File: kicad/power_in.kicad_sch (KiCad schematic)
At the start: 8 parts, among them J1 USB4105-GF-A, U1 CH224K

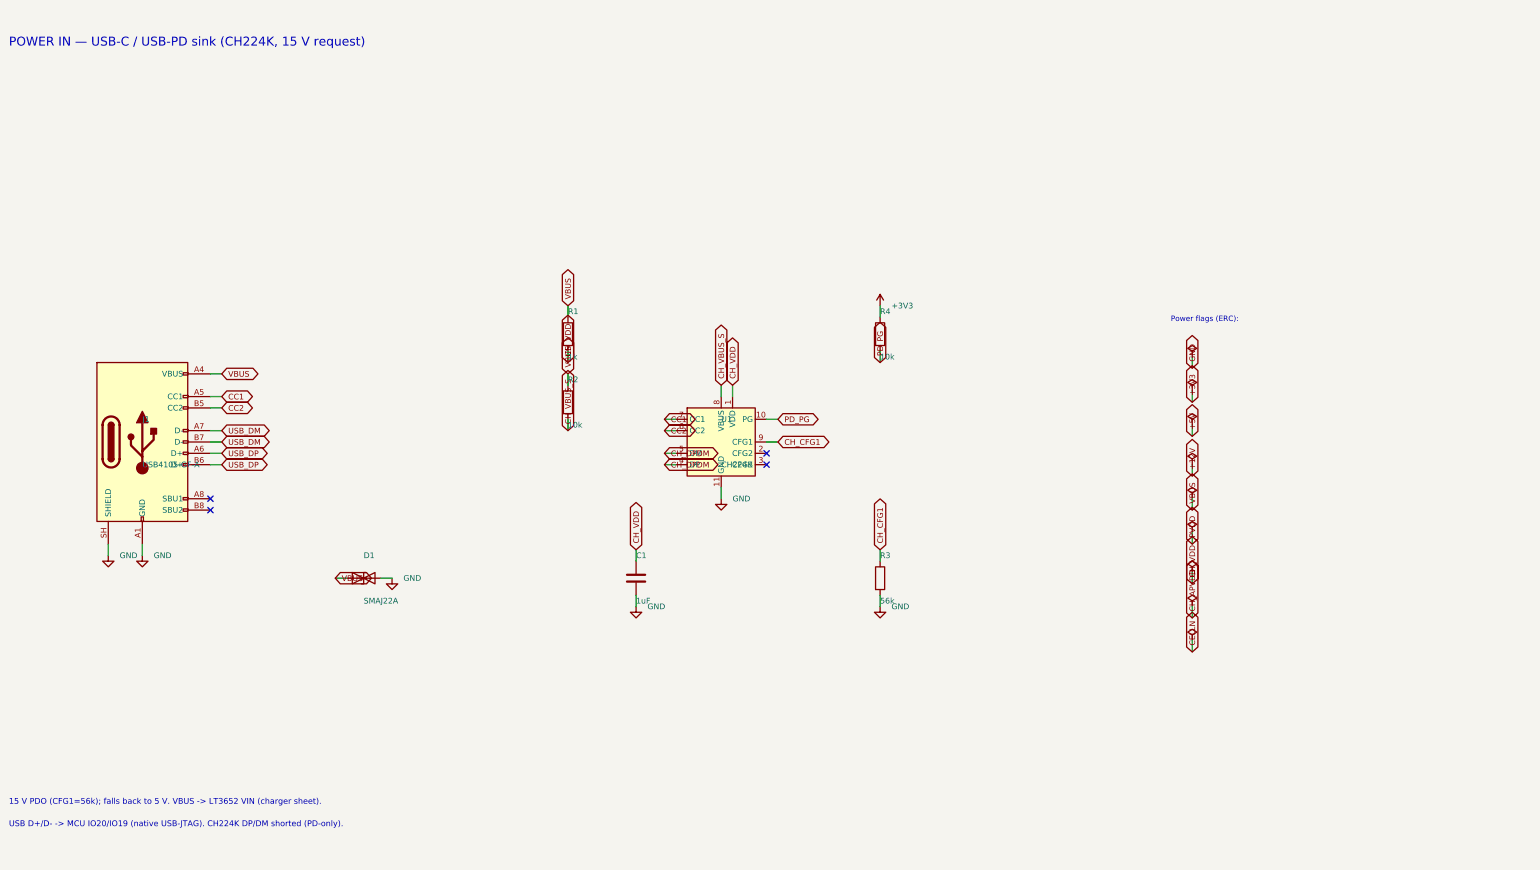
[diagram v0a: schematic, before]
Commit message: schematic second pass
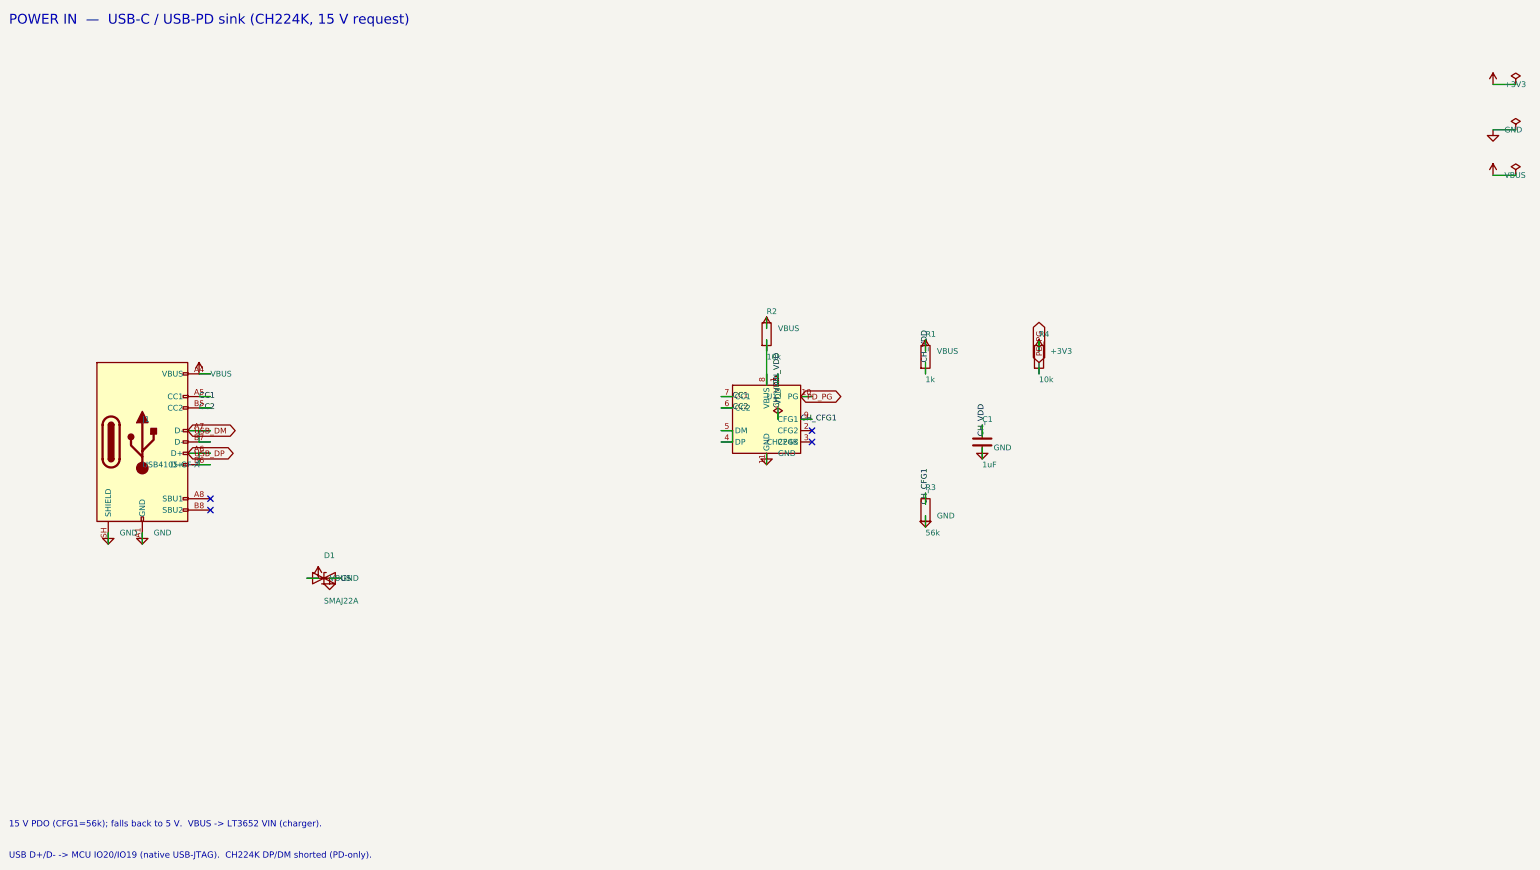
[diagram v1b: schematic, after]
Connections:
- net CH_DPDM: no longer names the net of U1.4 (DP), U1.5 (DM)
- net CH_VBUS_S: no longer names the net of R2.2, U1.8 (VBUS)
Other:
- note added: "15 V PDO (CFG1=56k); falls back to 5 V. VBUS -> LT3652 VIN (charger)."
- note removed: "15 V PDO (CFG1=56k); falls back to 5 V. VBUS -> LT3652 VIN (charger sheet)."
- note removed: "Power flags (ERC):"
